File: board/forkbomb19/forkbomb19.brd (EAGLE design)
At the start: 89.2 x 57 mm, 74 parts, among them T3 MMUN2133LT1G, U1 ESP-WROOM-03, U4 TPS61090RSAR, U5 MCP73871

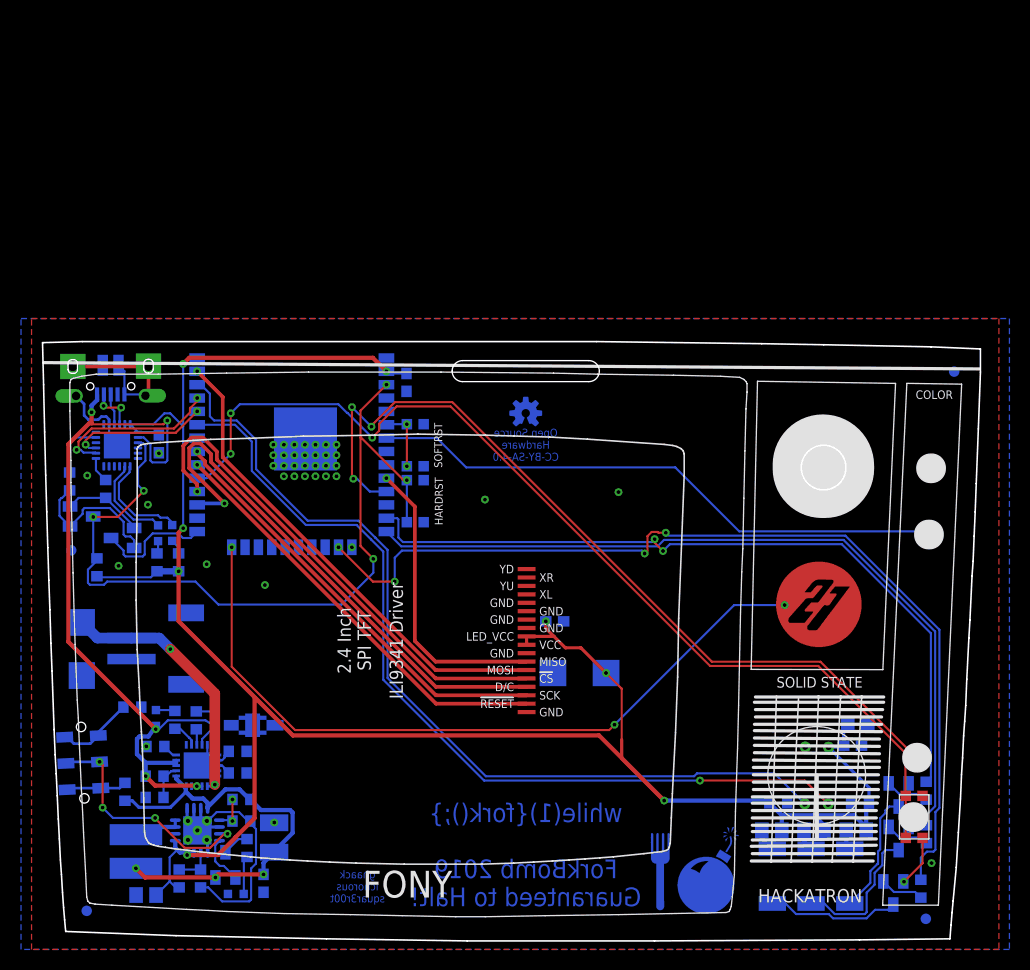
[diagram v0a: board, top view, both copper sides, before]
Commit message: ready for board sign off
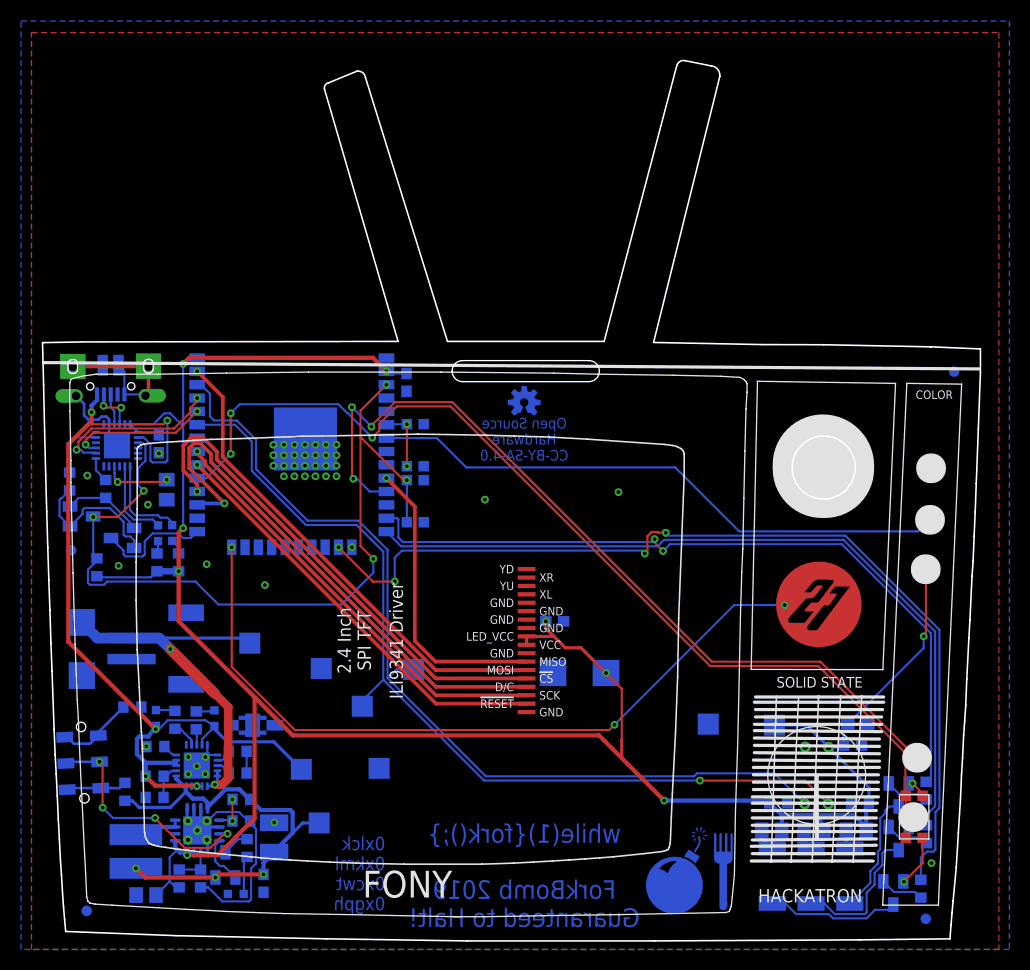
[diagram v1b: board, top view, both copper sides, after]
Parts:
- added 3V3_ROTARY: POT_GND, con-samtec:TSW-101-XX-G-S
- added C3: 4.7uF, rcl:C0805
- added TP_BATT_GND, TP_BATT_VBAT, TP_BATT_VLIPO, TP_I2C_GND, TP_I2C_SCL, TP_I2C_SDA, TP_PWR_3V3, TP_PWR_GND, TP_PWR_VBUS: TPSTP20SQ, testpad:TP20SQ
- moved ROTARY_A 1.40 mm to (84.6, 39.8)
- moved LOGO1 1.04 mm to (46.0, 51.0)
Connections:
- net TOUCH1 renamed TOUCH0
- new net I2C_GND: TP_I2C_GND.TP
- new net VPP: C3.1, U3.16
- net +3V3: now also 3V3_ROTARY.1, TP_PWR_3V3.TP
- net GND: now also C3.2, TP_BATT_GND.TP, TP_PWR_GND.TP
- net I2C_SCL: now also TP_I2C_SCL.TP
- net I2C_SDA: now also TP_I2C_SDA.TP
- net VBAT: now also TP_BATT_VBAT.TP
- net VBUS: now also TP_PWR_VBUS.TP
- net VLIPO: now also TP_BATT_VLIPO.TP
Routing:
- net +3V3: track 219.2 -> 243.1 mm, vias 8 -> 9
- net VLIPO: track 26.3 -> 39.2 mm
- net VBUS: track 77.3 -> 87.3 mm
- net VPP: track 0.00 -> 6.37 mm, vias 0 -> 2
- net GND: track 62.9 -> 67.7 mm, vias 41 -> 47
- net I2C_SDA: track 85.9 -> 89.3 mm
- net VBAT: track 44.9 -> 47.9 mm
- net I2C_SCL: track 86.3 -> 89.1 mm
- net N$19: track 9.78 -> 8.90 mm
- net N$20: track 8.79 -> 7.99 mm
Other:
- board size 89.2 x 57 mm -> 89.2 x 83.7 mm
- board text added: "+3V3"
- board text added: "+5V"
- board text added: "0xlck 0xkml 0xcwt 0xgph"
- board text added: "CUT HERE JUST FOR FUN"
- board text added: "GND"
- board text added: "ROTARY_3V3"
- board text added: "ROTARY_A"
- board text added: "ROTARY_B"
- board text added: "ROTARY_GND"
- board text added: "SCL"
- board text added: "SDA"
- board text added: "USER"
- board text added: "VBAT"
- board text added: "VLIPO"
- board text removed: "POT_GND"
- board text removed: "SOFTRST"
- board text removed: "ghaack ichorous squar3r00t"
